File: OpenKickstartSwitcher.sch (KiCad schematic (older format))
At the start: 14 parts, among them J1 Conn_01x03, J2 Conn_01x04, J99 OSHW_LOGO, U1 KS_SOCKET, U2 M27C160, U3 74LS04, U4 74LS08

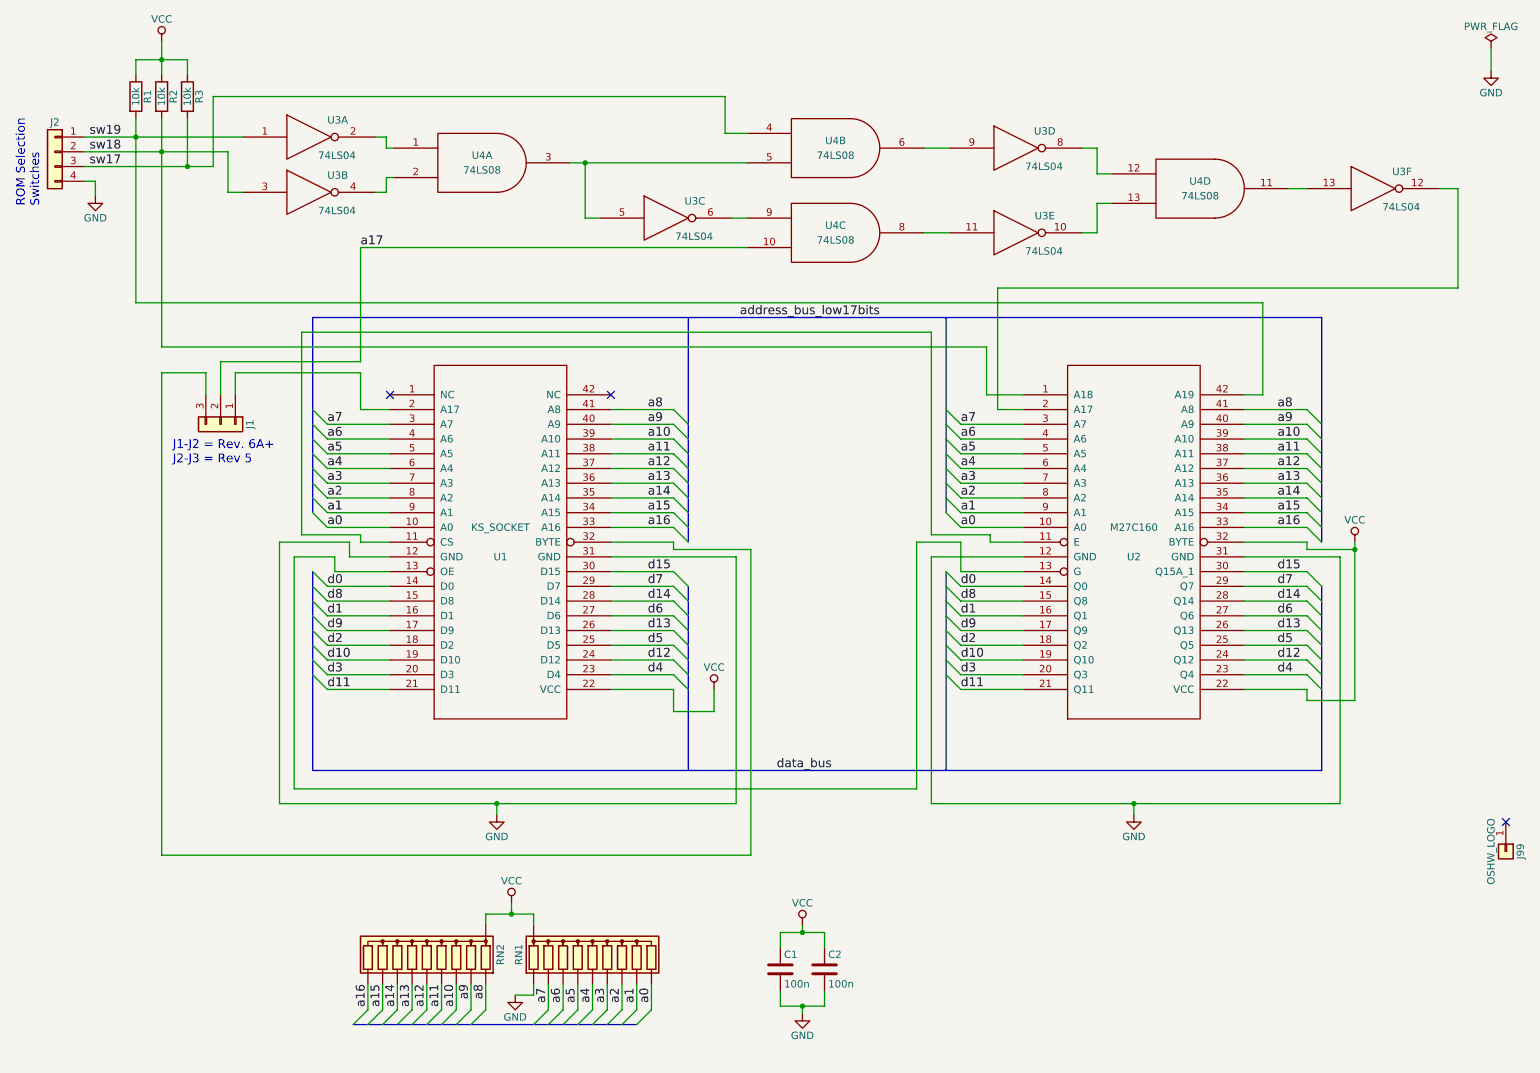
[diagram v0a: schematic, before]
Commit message: WIP
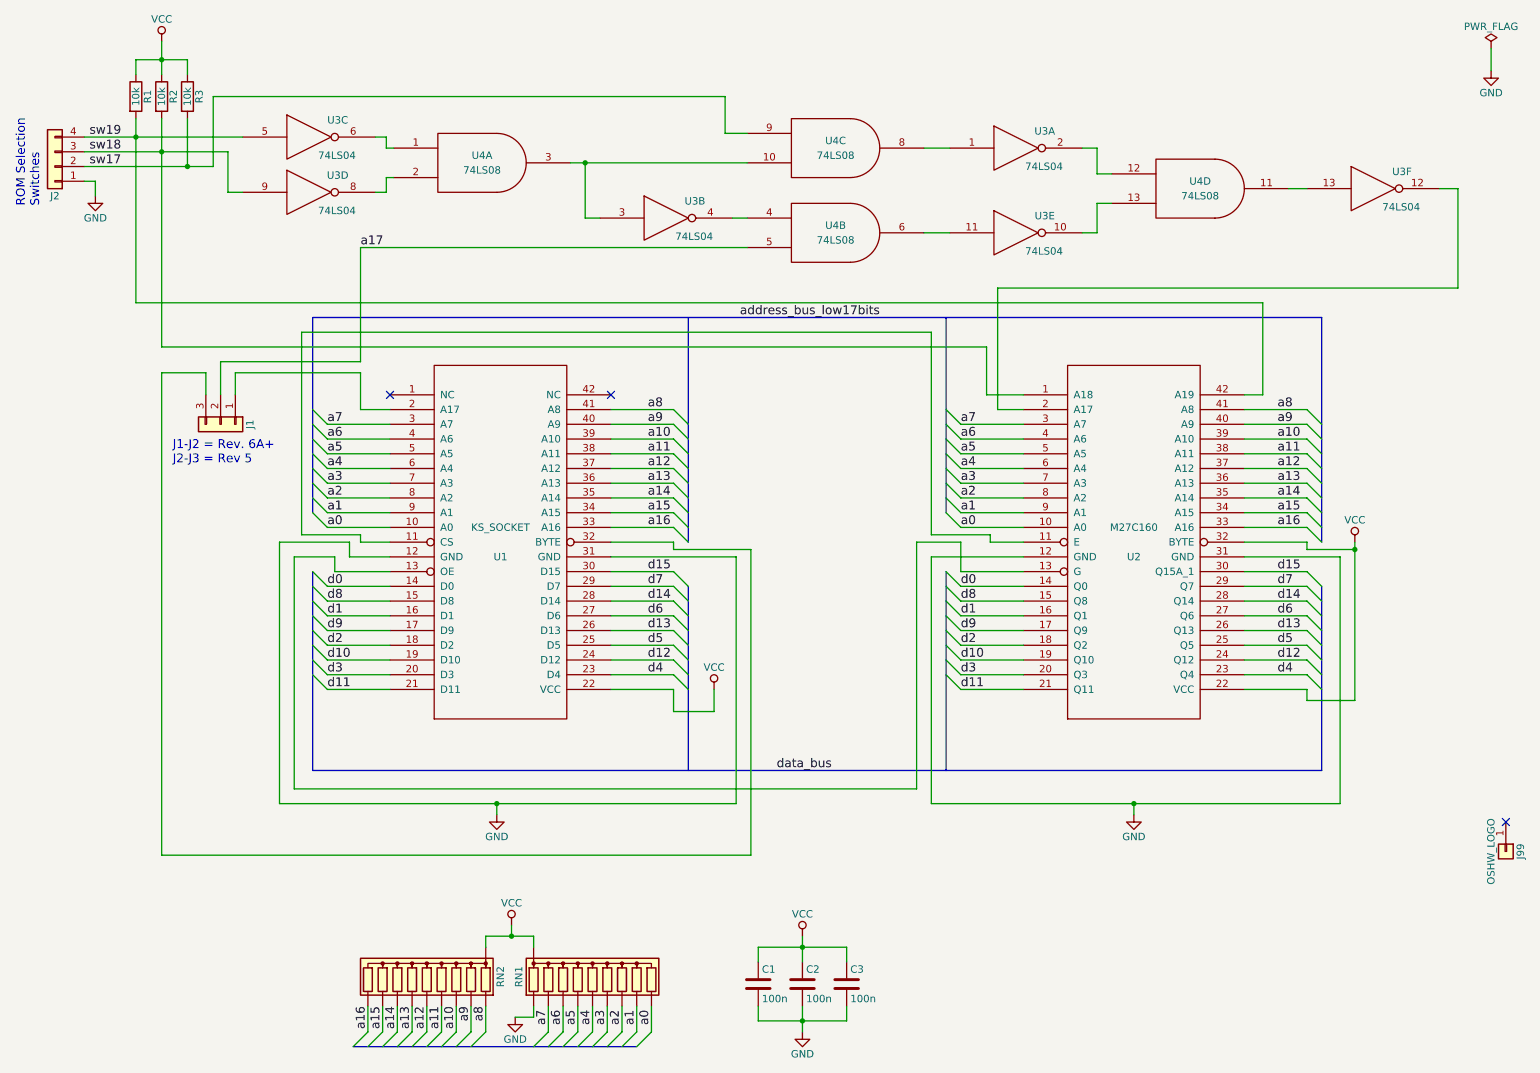
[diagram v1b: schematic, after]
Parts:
- added C3: 100n, Capacitors_THT:C_Disc_D7.0mm_W2.5mm_P5.00mm, symbol C
- J2: footprint (none) -> OpenKickstartSwitcher:LoosePads-4
- R1, R2, R3: footprint Resistors_THT:R_Axial_DIN0207_L6.3mm_D2.5mm_P10.16mm_Horizontal -> Resistors_THT:R_Axial_DIN0207_L6.3mm_D2.5mm_P7.62mm_Horizontal
- U2: footprint MODULE -> OpenKickstartSwitcher:DIP-42_Socket
- U3, U4: footprint (none) -> Housings_DIP:DIP-14_W7.62mm
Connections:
- net GND: now also J2.1 (Pin_1), C3.2; no longer J2.4 (Pin_4)
- net VCC: now also C3.1
- net a17: now also U4.5; no longer U4.10
- net sw17: now also J2.2 (Pin_2), U4.9; no longer J2.3 (Pin_3), U4.4
- net sw18: now also J2.3 (Pin_3), U3.9; no longer J2.2 (Pin_2), U3.3
- net sw19: now also J2.4 (Pin_4), U3.5; no longer J2.1 (Pin_1), U3.1
- net at U3.2: now also U4.12; no longer U4.1
- net at U3.4: now also U4.4; no longer U4.2
- net at U3.6: now also U4.1; no longer U4.9
- net at U3.8: now also U4.2; no longer U4.12
- net at U4.6: now also U3.11; no longer U3.9
- net at U4.8: now also U3.1; no longer U3.11
- new net: U3.3, U4.10, U4.3
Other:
- moved on the sheet: C1, C2, RN1, RN2, U3A, U3B, U3C, U3D, U4B, U4C
